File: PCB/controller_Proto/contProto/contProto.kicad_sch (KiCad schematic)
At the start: 42 parts, among them J1 Conn_01x05, J10 JST_1mm_3, J11 JST_1mm_3, J12 Conn_01x04, J13 Conn_01x02_Socket, J14 Conn_01x02_Socket, J15 Conn_01x04, J16 Conn_01x04, J2 Conn_01x04, J3 Conn_01x05, J4 Conn_01x04, J5 Conn_01x05, J6 Conn_01x05, J7 Conn_01x05, J8 Conn_01x05, J9 Conn_01x04, SW1 SMD_12x12mm_h8.5mm, SW10 SMD_12x12mm_h8.5mm, SW11 SMD_12x12mm_h8.5mm, SW12 SMD_12x12mm_h8.5mm, SW13 SMD_12x12mm_h8.5mm, SW14 SMD_12x12mm_h8.5mm, SW15 SMD_12x12mm_h8.5mm, SW16 SMD_12x12mm_h8.5mm, SW2 SMD_12x12mm_h8.5mm, SW3 SMD_12x12mm_h8.5mm, SW4 SMD_12x12mm_h8.5mm, SW5 SMD_12x12mm_h8.5mm, SW6 SMD_12x12mm_h8.5mm, SW7 SMD_12x12mm_h8.5mm, SW8 SMD_12x12mm_h8.5mm, SW9 SMD_12x12mm_h8.5mm, U1 ProMicroC, U2 ProMicroC, U3 DRV5033FAxLPG, U4 DRV5033FAxLPG

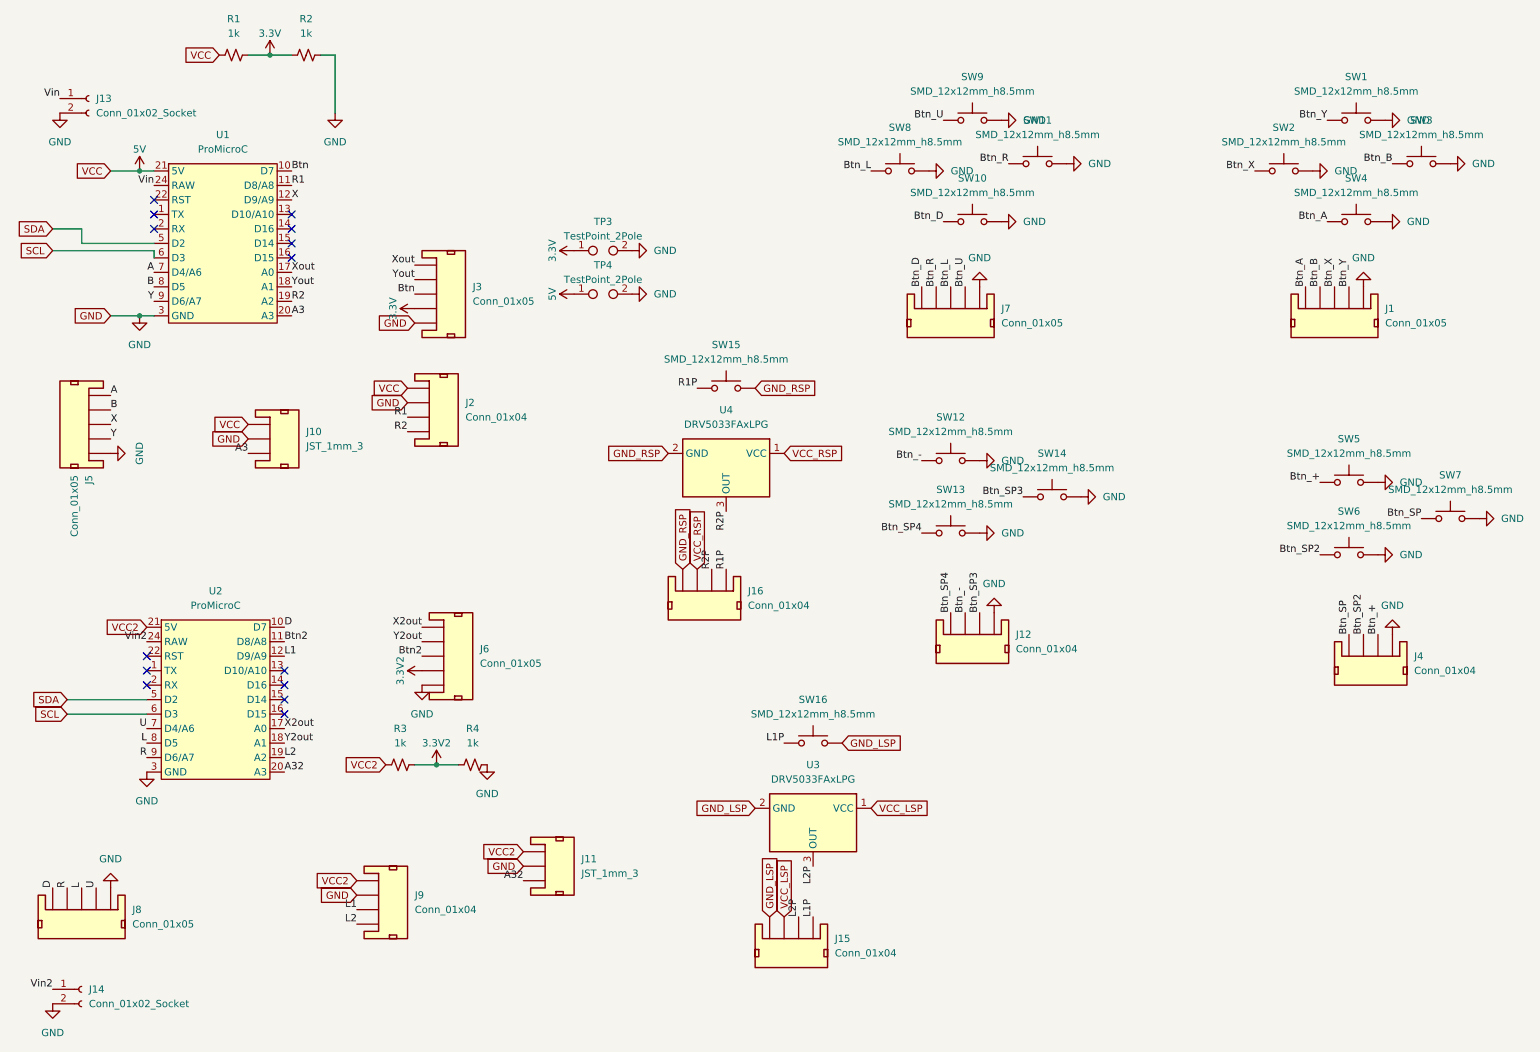
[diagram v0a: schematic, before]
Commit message: pcb fixing
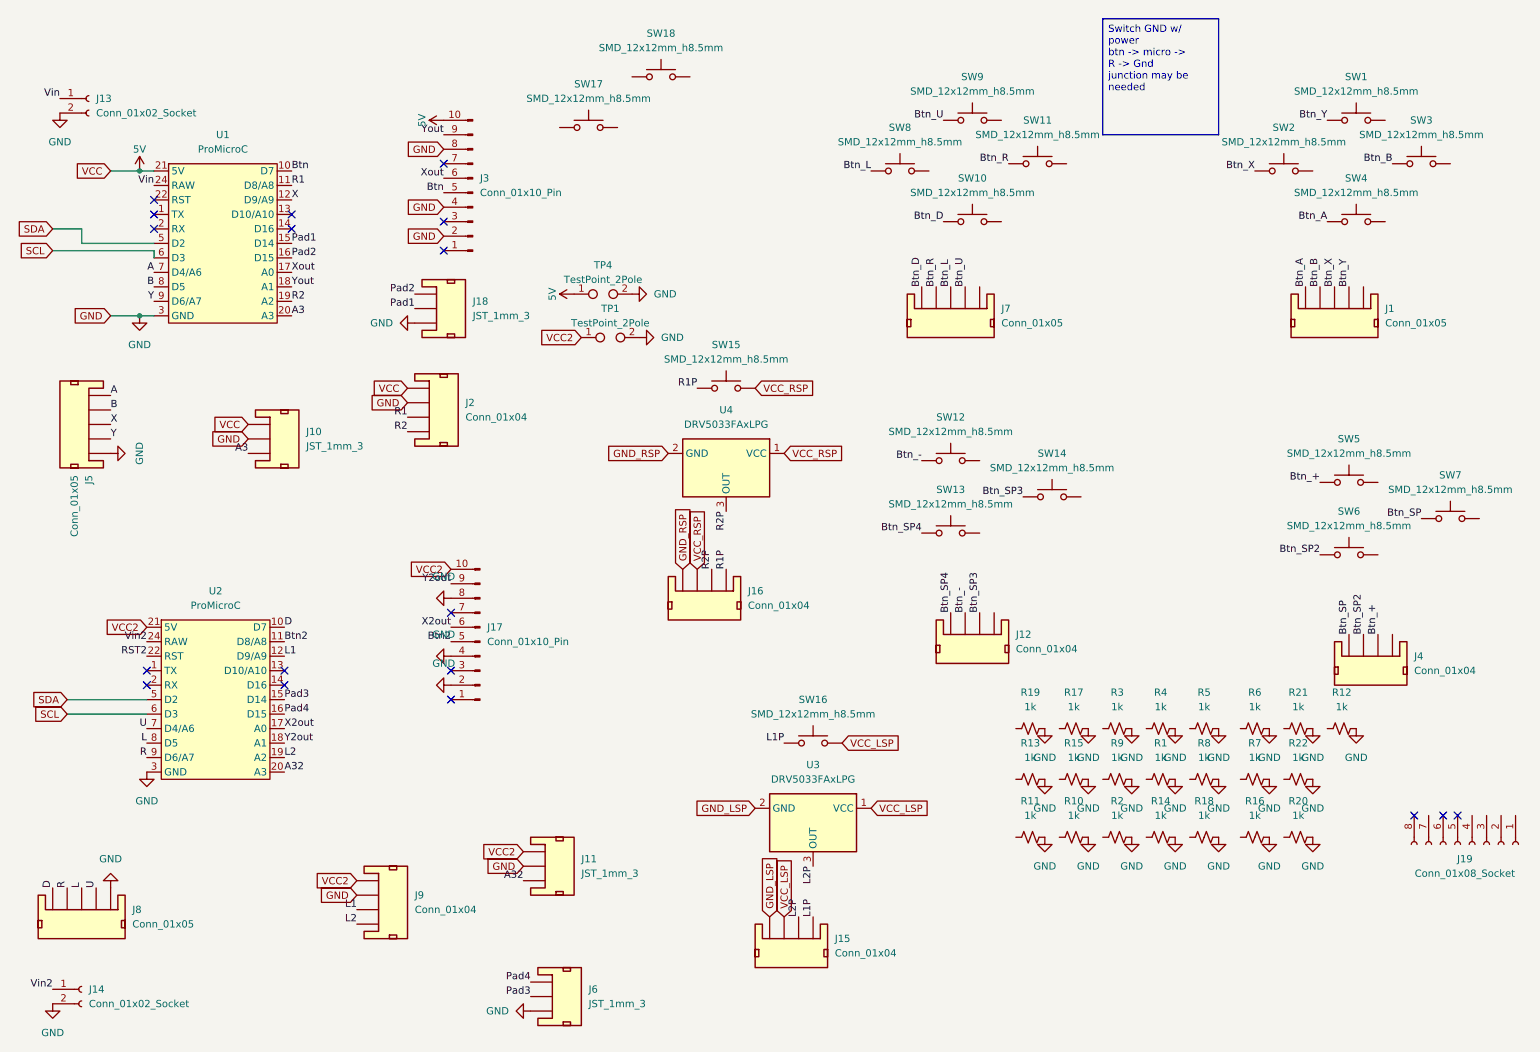
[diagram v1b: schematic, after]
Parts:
- removed J3, J6: Conn_01x05, PCM_SparkFun-Connector:JST_1x05_P1.25mm_Locking_Horizontal_SMD, symbol PCM_SparkFun-Connector:Conn_01x05_JST_P1.0mm_Horizontal_SMD
- removed TP3: TestPoint_2Pole, TestPoint:TestPoint_Bridge_Pitch2.0mm_Drill0.7mm, symbol Connector:TestPoint_2Pole
- added J17, J3: Conn_01x10_Pin, Connector_FFC-FPC:Amphenol_F32Q-1A7x1-11010_1x10-1MP_P0.5mm_Horizontal, symbol Connector:Conn_01x10_Pin
- added J18, J6: JST_1mm_3, PCM_SparkFun-Connector:JST_1x03_P1.0mm_Horizontal_SMD, symbol PCM_SparkFun-Connector:Conn_01x03_JST_P1.0mm_Horizontal_SMD
- added J19: Conn_01x08_Socket, Connector_PinSocket_1.00mm:PinSocket_1x08_P1.00mm_Vertical, symbol Connector:Conn_01x08_Socket
- added R10, R11, R12, R13, R14, R15, R16, R17, R18, R19, R20, R21, R22, R5, R6, R7, R8, R9: 1k, PCM_SparkFun-Resistor:R_0402_1005Metric, symbol PCM_SparkFun-Resistor:1k_0402
- added SW17, SW18: SMD_12x12mm_h8.5mm, Button_Switch_SMD:SW_Tactile_SPST_NO_Straight_CK_PTS636Sx25SMTRLFS, symbol PCM_SparkFun-Switch:SPST_Push_SMD_12x12mm_h8.5mm
- added TP1: TestPoint_2Pole, TestPoint:TestPoint_Bridge_Pitch2.0mm_Drill0.7mm, symbol Connector:TestPoint_2Pole
- J12, J15, J16, J2, J4, J9: footprint PCM_SparkFun-Connector:JST_1x04_P2.0mm_Horizontal_SMD -> PCM_SparkFun-Connector:JST_1x04_P1.25mm_Locking_Horizontal_SMD
- J13, J14: footprint (none) -> Connector_PinSocket_1.00mm:PinSocket_1x02_P1.00mm_Vertical
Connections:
- net 5V: now also J3.10 (Pin_10); no longer R1.1
- net Btn: now also J3.5 (Pin_5)
- net Btn2: now also J17.5 (Pin_5)
- net GND: now also R1.2, R3.2, J17.2 (Pin_2), J17.4 (Pin_4), J17.8 (Pin_8), J18.3, J3.2 (Pin_2), J3.4 (Pin_4), J3.8 (Pin_8), J6.3, R10.2, R11.2, R12.2, R13.2, R14.2, R15.2, R16.2, R17.2, R18.2, R19.2, R20.2, R21.2, R22.2, R5.2, R6.2, R7.2, R8.2, R9.2, TP1.2; no longer J1.1, J12.1, J4.1, J7.1, SW1.2, SW10.2, SW11.2, SW12.2, SW13.2, SW14.2, SW2.2, SW3.2, SW4.2, SW5.2, SW6.2, SW7.2, SW8.2, SW9.2
- net GND_LSP: no longer SW16.2
- net GND_RSP: no longer SW15.2
- net VCC2: now also J17.10 (Pin_10), TP1.1; no longer R3.1
- net VCC_LSP: now also SW16.2
- net VCC_RSP: now also SW15.2
- net X2out: now also J17.6 (Pin_6)
- net Xout: now also J3.6 (Pin_6)
- net Y2out: now also J17.9 (Pin_9)
- net Yout: now also J3.9 (Pin_9)
- net Pad3: now reaches U2.15 (D14)
- net Pad3: now also J6.2
- net Pad4: now reaches U2.16 (D15)
- net Pad4: now also J6.1
- net RST2: now reaches U2.22 (RST)
- net Pad1: now reaches U1.15 (D14)
- net Pad1: now also J18.2
- net Pad2: now reaches U1.16 (D15)
- net Pad2: now also J18.1
- net 3.3V: no longer names the net of R2.1
- net 3.3V: no longer R1.2
- net 3.3V2: no longer names the net of R4.1
- net 3.3V2: no longer R3.2
- no-connect marks 14 -> 18
